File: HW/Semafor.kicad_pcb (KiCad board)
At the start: 2 copper layers, 100 x 100 mm, 92 parts, among them J1 USB_C_Receptacle_USB2.0, J3 Conn_01x03_Male, M1 Motor_DC, Q1 Q_NMOS_GSD, Q2 Q_PMOS_GSD, Q3 Q_NMOS_GSD, Q4 Q_NMOS_GSD, Q5 Q_Photo_NPN, SW6 SW_SPDT, U1 ESP32-C3, U2 CN3058E, U3 LT1930, U4 E22-900T22D, U5 AT42QT1070-S

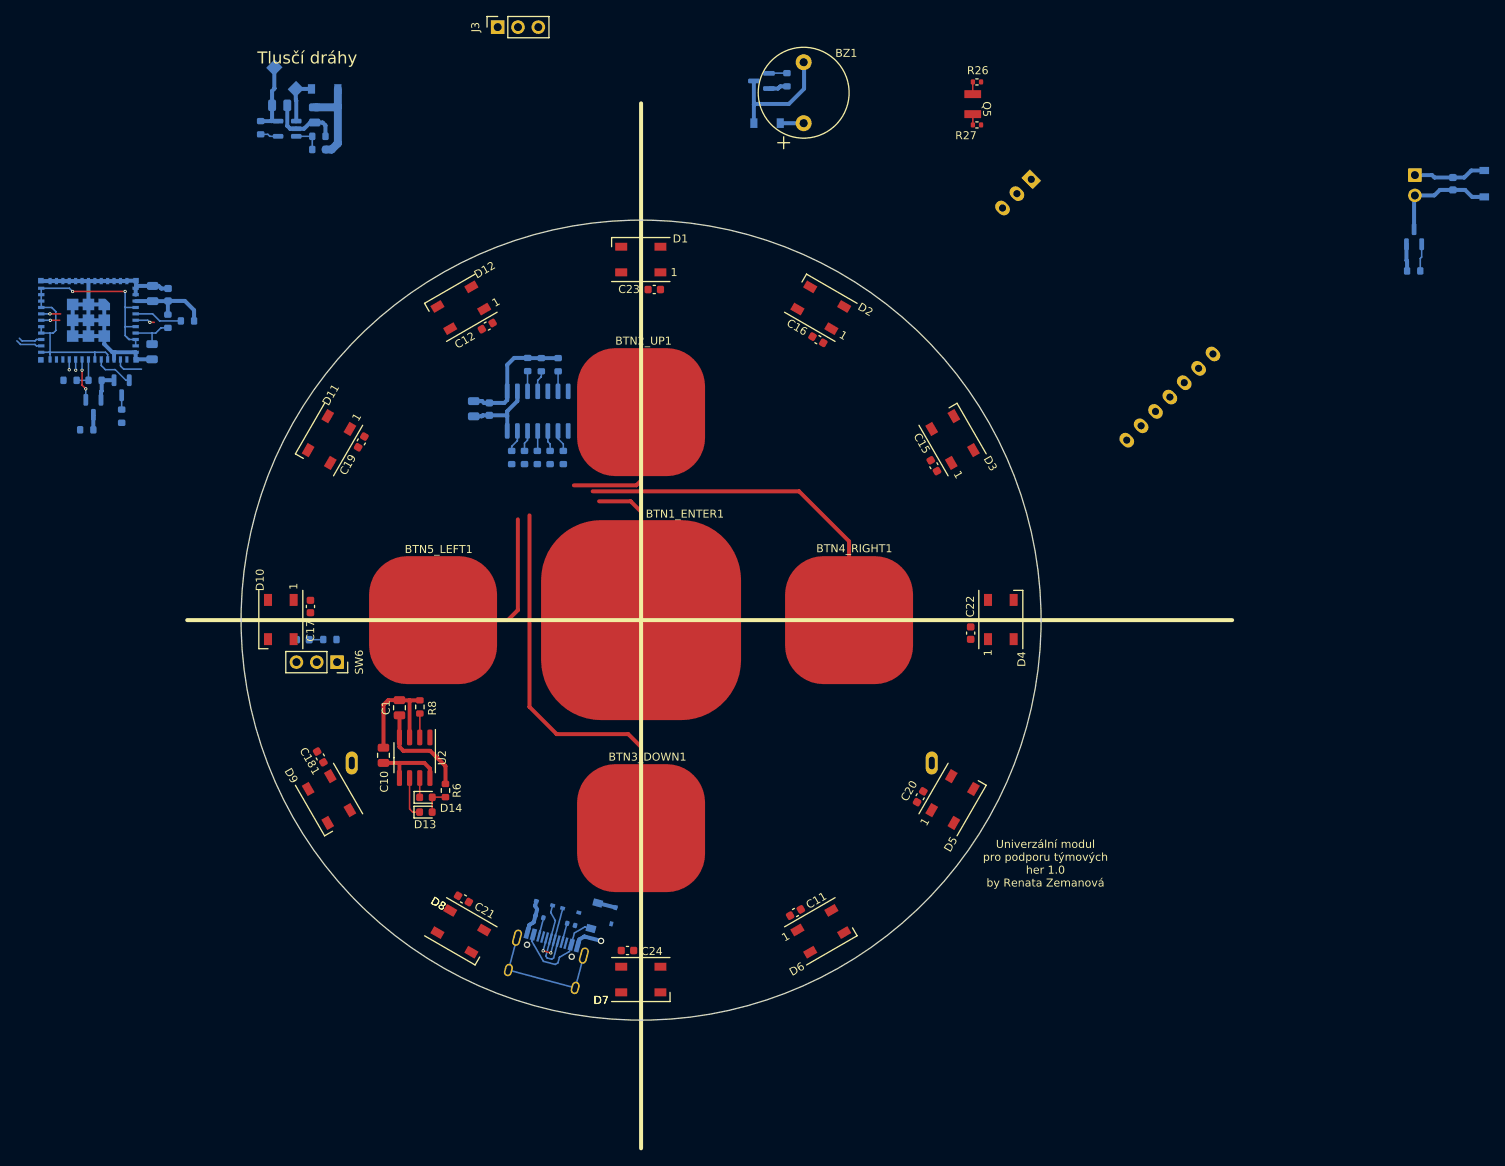
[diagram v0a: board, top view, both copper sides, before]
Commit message: done routing of version 1.0
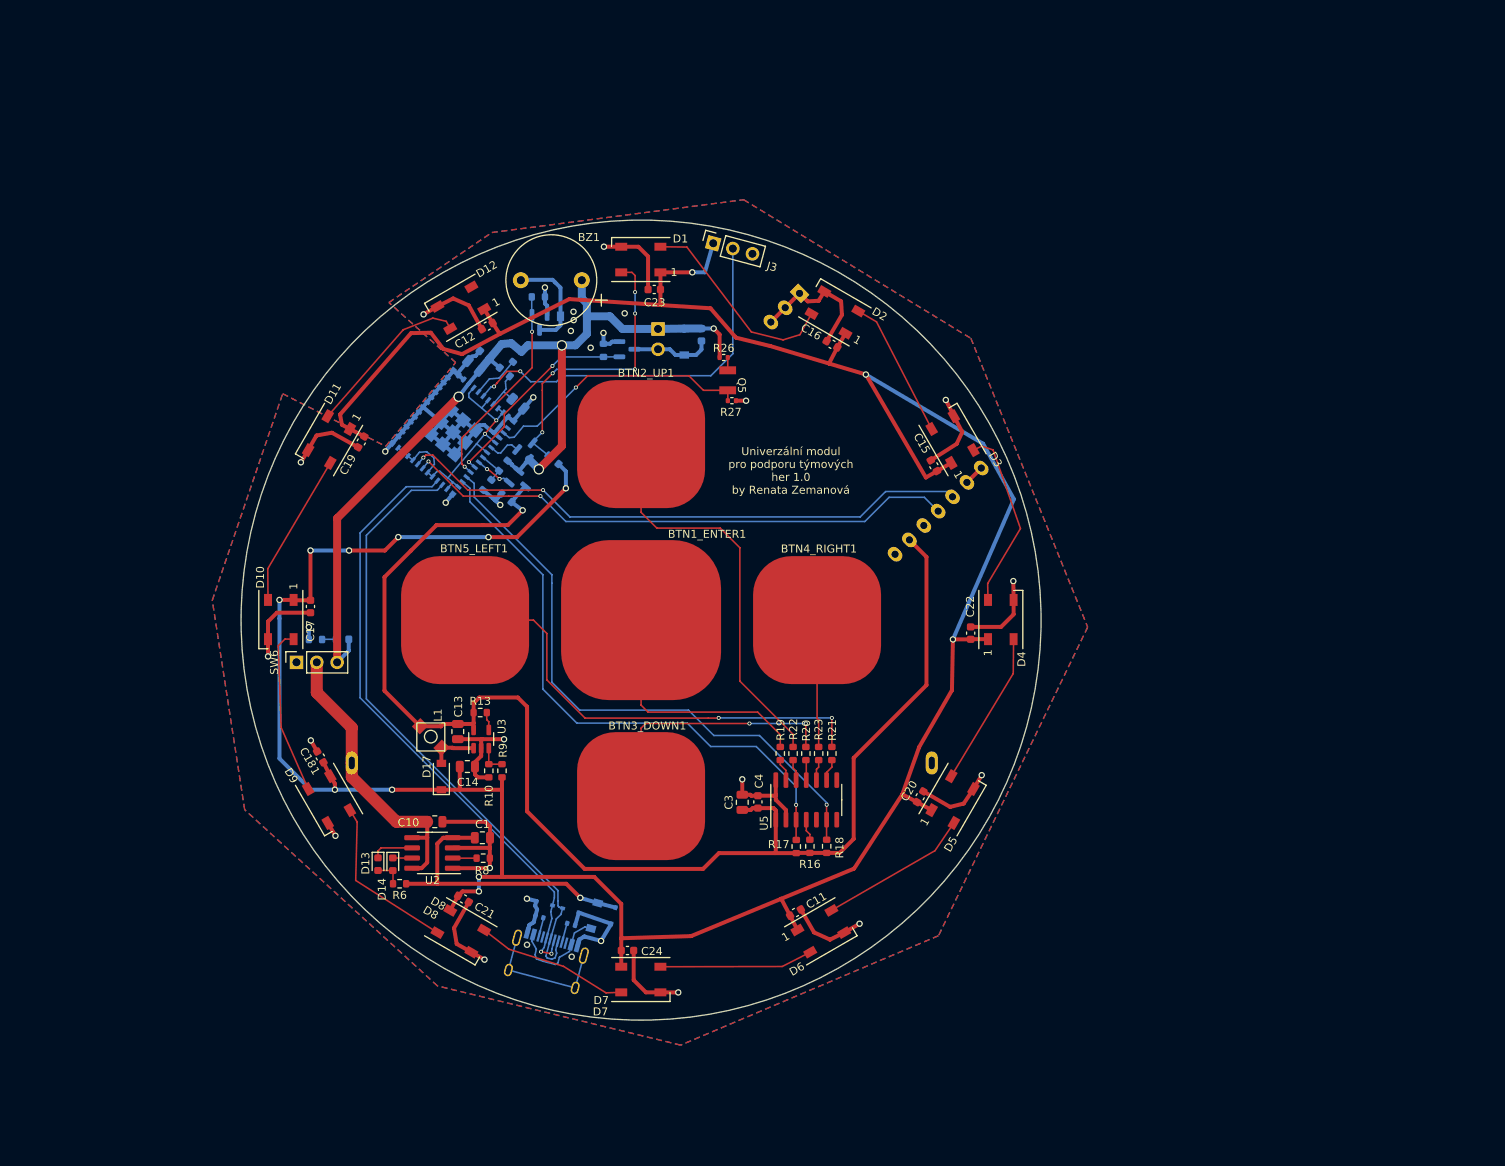
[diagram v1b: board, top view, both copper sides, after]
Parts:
- BTN1_ENTER1: footprint Library:Cap_btn_2,5x2,5 -> Library:Cap_btn_2x2
- C13, C14, C3, C4, D17, L1, R10, R13, R16, R17, R18, R19, R20, R21, R22, R23, R9, U3, U5: moved to F.Cu
- moved BTN1_ENTER1 409.9 mm to (100.0, 100.0)
- moved D22 101.9 mm to (105.4, 65.2)
- moved R15 101.8 mm to (95.3, 66.3), turned to 90 degrees
- moved Q4 99.4 mm to (98.2, 66.1), turned to 0 degrees
- moved M1 96.5 mm to (102.1, 63.6)
- moved C25 95.8 mm to (107.5, 64.3)
- moved D17 87.2 mm to (75.0, 119.6), turned to 90 degrees
- moved L1 84.3 mm to (73.7, 114.6), turned to 0 degrees
- moved C14 83.7 mm to (78.3, 118.3), turned to 0 degrees
- moved R10 82.1 mm to (81.0, 118.8), turned to -90 degrees
- moved C13 81.4 mm to (77.1, 113.9), turned to -90 degrees
- moved R9 81.0 mm to (82.6, 118.8), turned to 90 degrees
- moved U3 80.1 mm to (80.0, 114.9), turned to 90 degrees
- moved R13 78.1 mm to (79.9, 111.6), turned to 0 degrees
- moved R17 69.0 mm to (119.4, 128.3), turned to 90 degrees
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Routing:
- net PWR_LED: track 11.6 -> 390.9 mm, vias 0 -> 13
- net GND: track 101.8 -> 256.5 mm, vias 1 -> 30
- net 3V3_SWITCHED: track 26.5 -> 173.5 mm, vias 0 -> 1
- net +3V3: track 27.1 -> 114.9 mm, vias 0 -> 4
- net SCL: track 2.50 -> 75.3 mm, vias 0 -> 1
- net SDA: track 2.53 -> 73.5 mm, vias 0 -> 1
- net RX_LoRa: track 2.43 -> 72.1 mm, vias 1 -> 2
- net TX_LoRa: track 2.32 -> 69.9 mm, vias 1 -> 2
- net D+: track 11.4 -> 78.2 mm
- net D-: track 13.3 -> 79.0 mm
- net DATA_LED_SIDE: track 2.43 -> 47.7 mm, vias 1 -> 2
- net Net-(BTN5_LEFT1-Pad1): track 22.5 -> 58.0 mm, vias 0 -> 2
- net DATA_LED_OUT: track 1.80 -> 36.4 mm, vias 0 -> 5
- net Net-(BTN2_UP1-Pad1): track 17.2 -> 50.4 mm
- net Net-(BTN4_RIGHT1-Pad1): track 44.5 -> 15.9 mm
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- added copper zone on B.Cu, net GND
- added copper zone on F.Cu, net GND
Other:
- board text removed: "Tlusčí dráhy"
